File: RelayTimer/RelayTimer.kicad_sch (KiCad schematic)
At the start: 21 parts, among them J1 Jack-DC, J2 Relay_Con, Q1 2N3904, SW1 SW_Push, U1 ATtiny85-20P

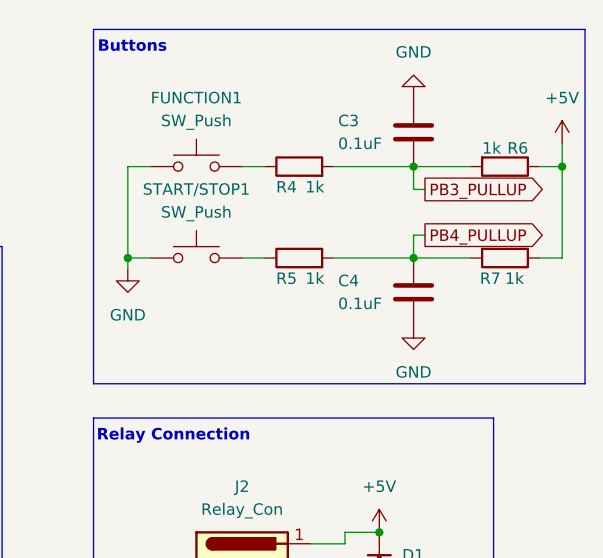
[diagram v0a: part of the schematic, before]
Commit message: fixed small issue and updated board
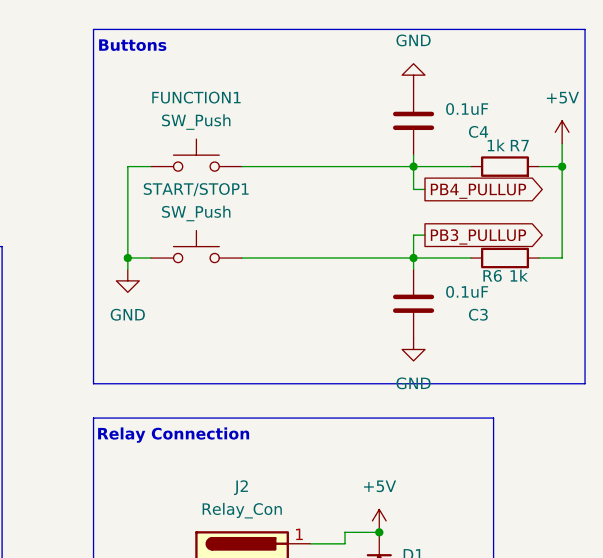
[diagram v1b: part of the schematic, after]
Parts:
- removed R4, R5: 1k, Resistor_THT:R_Axial_DIN0204_L3.6mm_D1.6mm_P2.54mm_Vertical, symbol Device:R
- R6, R7: footprint Resistor_THT:R_Axial_DIN0204_L3.6mm_D1.6mm_P2.54mm_Vertical -> Resistor_THT:R_Axial_DIN0204_L3.6mm_D1.6mm_P7.62mm_Horizontal
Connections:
- net +5V: now also R6.2, R7.2; no longer R6.1, R7.1
- net PB3_PULLUP: now also R6.1, START/STOP1.2; no longer R6.2
- net PB4_PULLUP: now also FUNCTION1.2, R7.1; no longer R7.2
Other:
- moved on the sheet: C3, C4, R6, R7
